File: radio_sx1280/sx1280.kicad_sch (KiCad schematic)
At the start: 19 parts, among them J1 Conn_01x08, J2 Conn_01x08, U1 TG-5006Cx, U2 SX1280, U3 2450FM07D0034

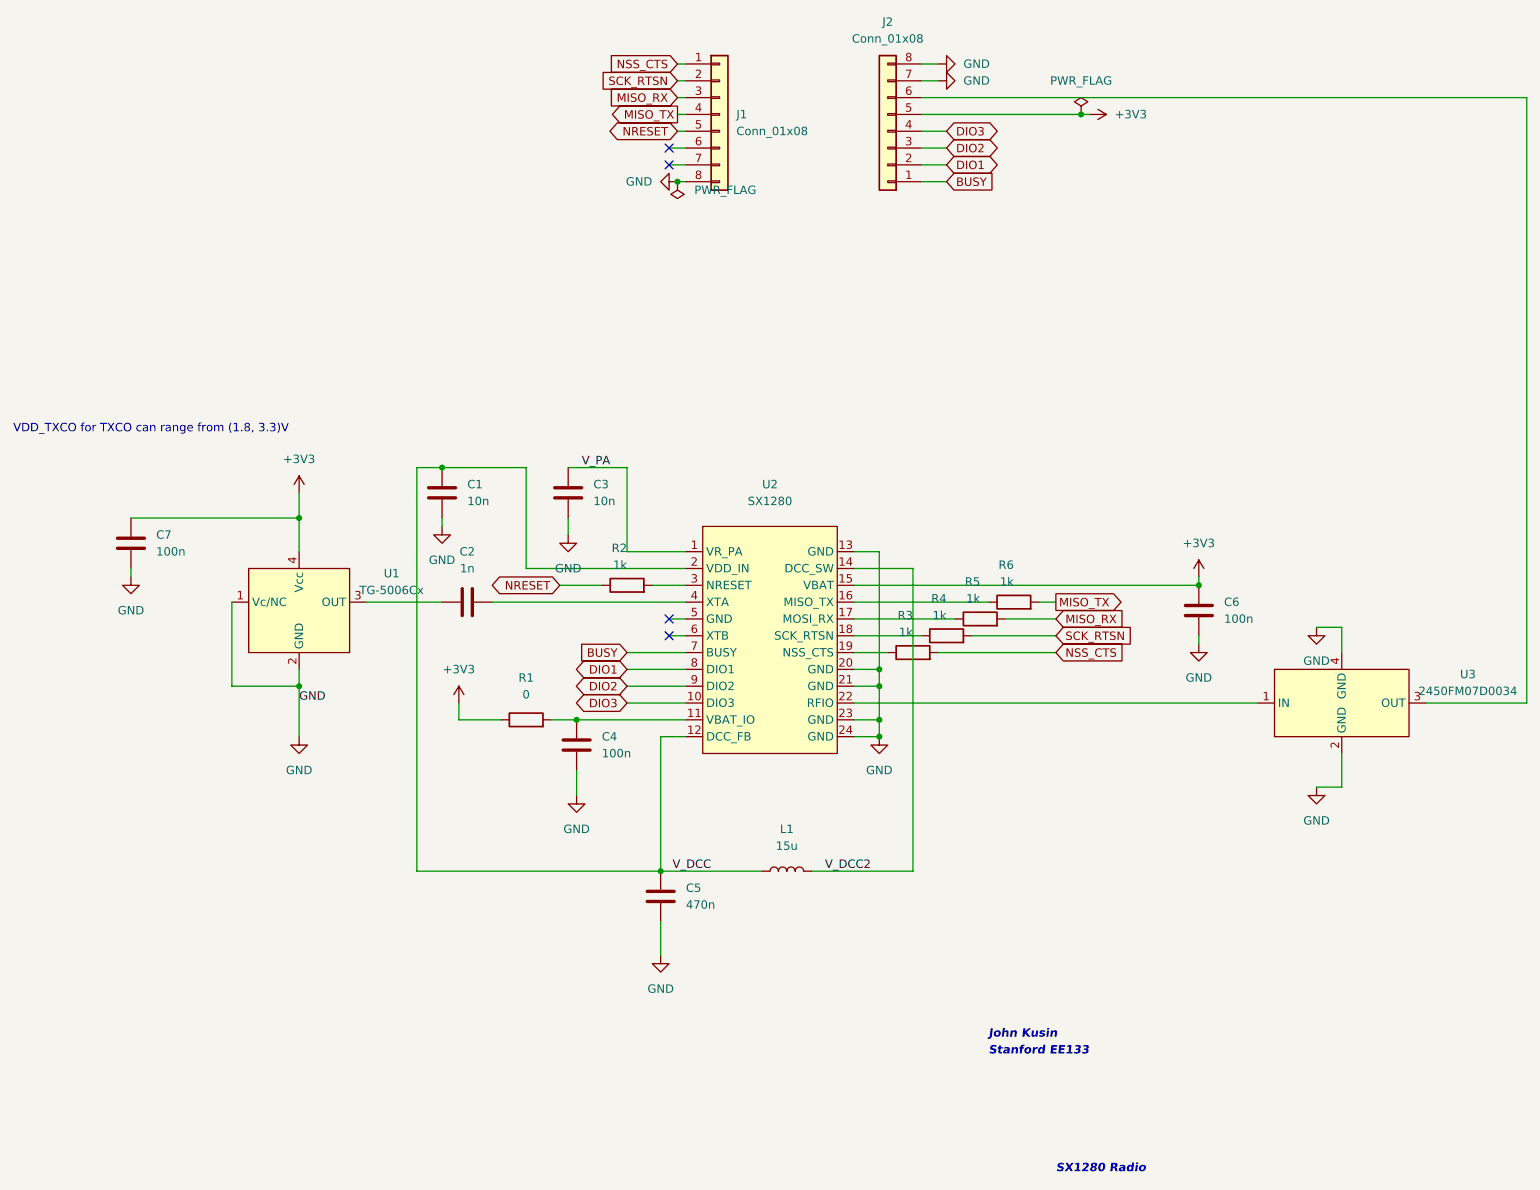
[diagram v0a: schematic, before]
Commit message: schematic and layout
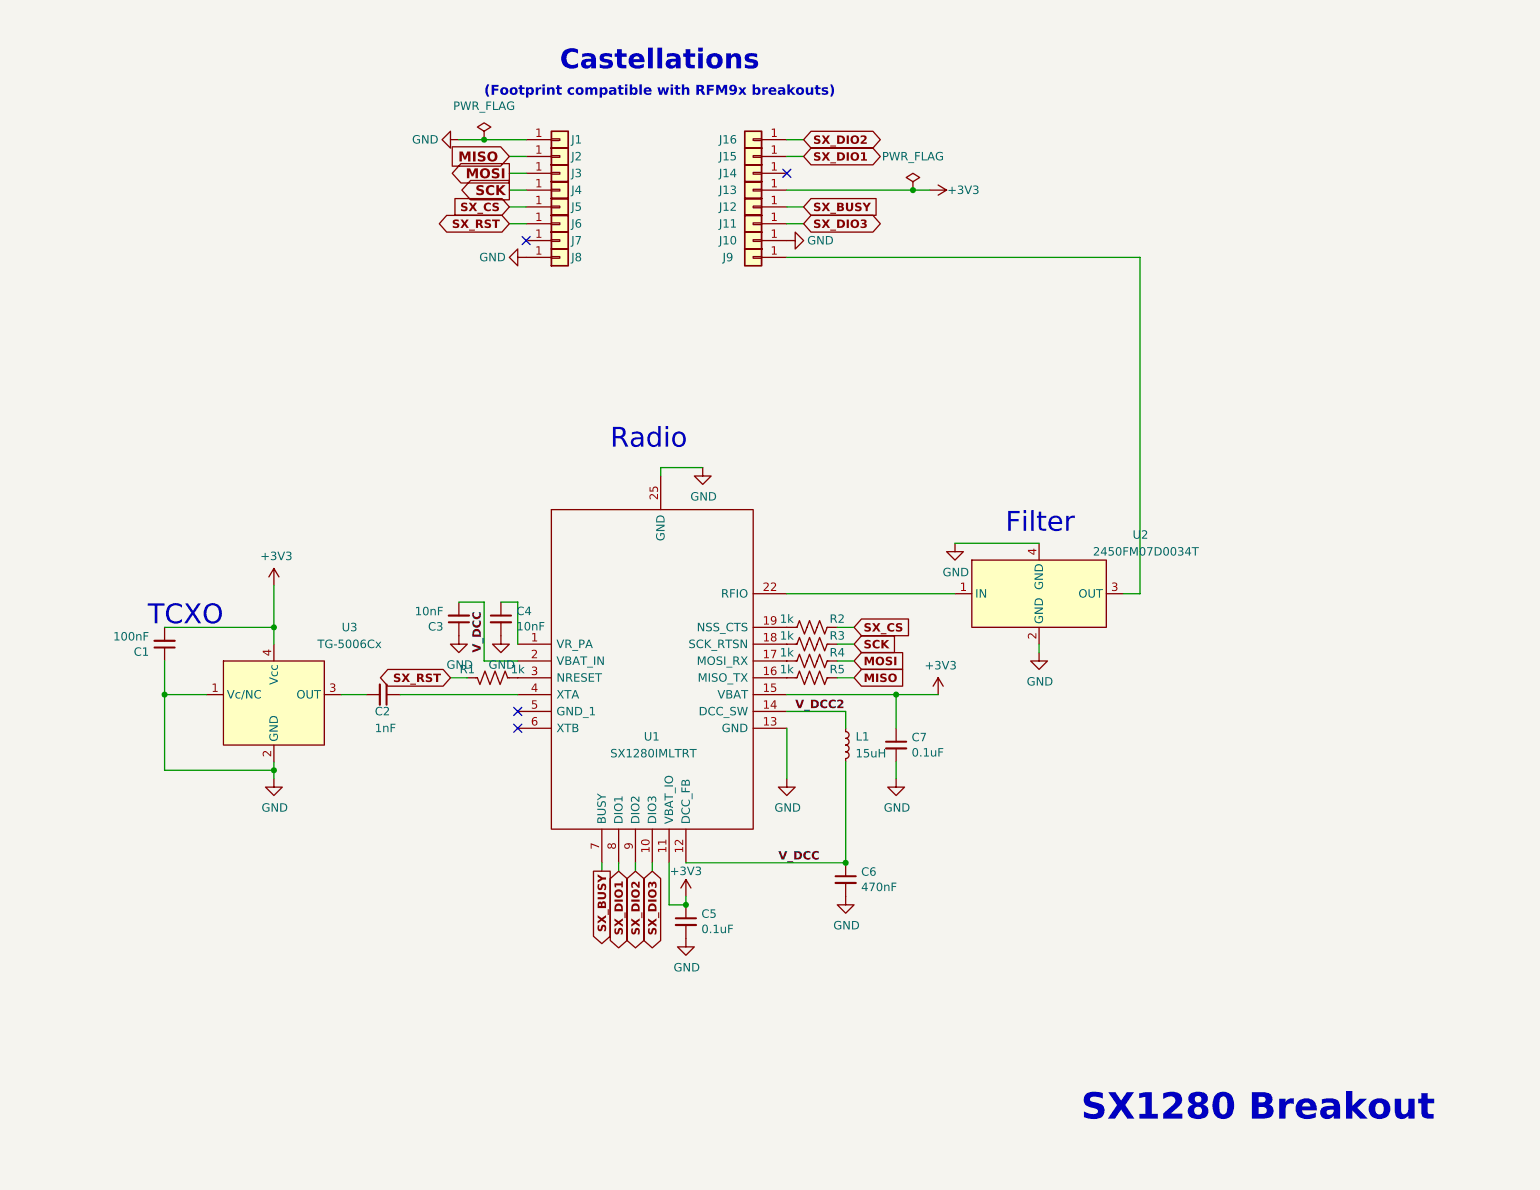
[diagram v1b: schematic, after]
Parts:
- removed C1, C3: 10n, symbol Device:C
- removed C2: 1n, symbol Device:C
- removed C4, C6, C7: 100n, symbol Device:C
- removed C5: 470n, symbol Device:C
- removed J1, J2: Conn_01x08, symbol Connector_Generic:Conn_01x08
- removed L1: 15u, symbol Device:L
- removed R1: 0, symbol Device:R
- removed R2, R3, R4, R5, R6: 1k, symbol Device:R
- removed U1: TG-5006Cx, symbol Oscillator:TG-5006Cx
- removed U2: SX1280, symbol semtech:SX1280
- removed U3: 2450FM07D0034, symbol RF_Filter:2450FM07D0034
- added C1: 100nF, Capacitor_SMD:C_0402_1005Metric, symbol Device:C_Small
- added C2: 1nF, Capacitor_SMD:C_0402_1005Metric, symbol Device:C_Small
- added C3, C4: 10nF, Capacitor_SMD:C_0402_1005Metric, symbol Device:C_Small
- added C5, C7: 0.1uF, Capacitor_SMD:C_0402_1005Metric, symbol Device:C_Small
- added C6: 470nF, Capacitor_SMD:C_0402_1005Metric, symbol Device:C_Small
- added J1, J10, J11, J12, J13, J14, J15, J16, J2, J3, J4, J5, J6, J7, J8, J9: Conn_01x01, custom-footprints:castellated, symbol Connector_Generic:Conn_01x01
- added L1: 15uH, Inductor_SMD:L_0805_2012Metric, symbol Device:L_Small
- added R1, R2, R3, R4, R5: 1k, Resistor_SMD:R_0402_1005Metric, symbol Device:R_US
- added U1: SX1280IMLTRT, custom-footprints:QFN50P400X400X80-25N-D, symbol symbols:SX1280IMLTRT
- added U2: 2450FM07D0034T, custom-footprints:2450FM07D0034T, symbol RF_Filter:2450FM07D0034
- added U3: TG-5006Cx, Crystal:Crystal_SMD_2520-4Pin_2.5x2.0mm, symbol Oscillator:TG-5006Cx
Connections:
- net +3V3: now also C1.2, C5.1, C7.1, J13.1 (Pin_1), U1.11 (VBAT_IO), U1.15 (VBAT), U3.4 (Vcc)
- net GND: now also C1.1, C3.1, C4.2, C5.2, C6.2, C7.2, J1.1 (Pin_1), J10.1 (Pin_1), J8.1 (Pin_1), U1.13 (GND), U1.20 (GND), U1.21 (GND), U1.23 (GND), U1.24 (GND), U1.25 (GND), U2.2 (GND), U2.4 (GND), U3.1 (Vc/NC), U3.2 (GND)
- net V_DCC: now also C3.2, C6.1, L1.2, U1.12 (DCC_FB), U1.2 (VBAT_IN)
- net V_DCC2: now also L1.1, U1.14 (DCC_SW)
- new net: U1.22 (RFIO), U2.1 (IN)
- new net: J9.1 (Pin_1), U2.3 (OUT)
- new net: C4.1, U1.1 (VR_PA)
- new net: R5.2, U1.16 (MISO_TX)
- new net: R4.2, U1.17 (MOSI_RX)
- new net: R3.2, U1.18 (SCK_RTSN)
- new net: R2.2, U1.19 (NSS_CTS)
- new net: R1.2, U1.3 (NRESET)
- new net: C2.1, U1.4 (XTA)
- new net: C2.2, U3.3 (OUT)
- new net MISO: J2.1 (Pin_1), R5.1
- new net MOSI: J3.1 (Pin_1), R4.1
- new net SCK: J4.1 (Pin_1), R3.1
- new net SX_BUSY: J12.1 (Pin_1), U1.7 (BUSY)
- new net SX_CS: J5.1 (Pin_1), R2.1
- new net SX_DIO1: J15.1 (Pin_1), U1.8 (DIO1)
- new net SX_DIO2: J16.1 (Pin_1), U1.9 (DIO2)
- new net SX_DIO3: J11.1 (Pin_1), U1.10 (DIO3)
- new net SX_RST: J6.1 (Pin_1), R1.1
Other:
- note added: "(Footprint compatible with RFM9x breakouts)"
- note added: "Castellations"
- note added: "Filter"
- note added: "Radio"
- note added: "SX1280 Breakout"
- note added: "TCXO"
- note removed: "John Kusin"
- note removed: "SX1280 Radio"
- note removed: "Stanford EE133"
- note removed: "VDD_TXCO for TXCO can range from (1.8, 3.3)V"
- company: (none) -> Stanford University
- title: (none) -> EE 133 Analog Communications Design Laboratory
